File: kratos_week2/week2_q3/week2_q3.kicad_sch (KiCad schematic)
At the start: 17 parts, among them J1 XT60-M, J10 XT60-M, J11 XT60-M, J2 XT60-M, J3 XT60-M, J4 XT60-M, J5 XT60-M, J6 XT60-M, J7 Conn_01x02_Pin, J8 Conn_01x02_Pin, J9 Conn_01x02_Pin

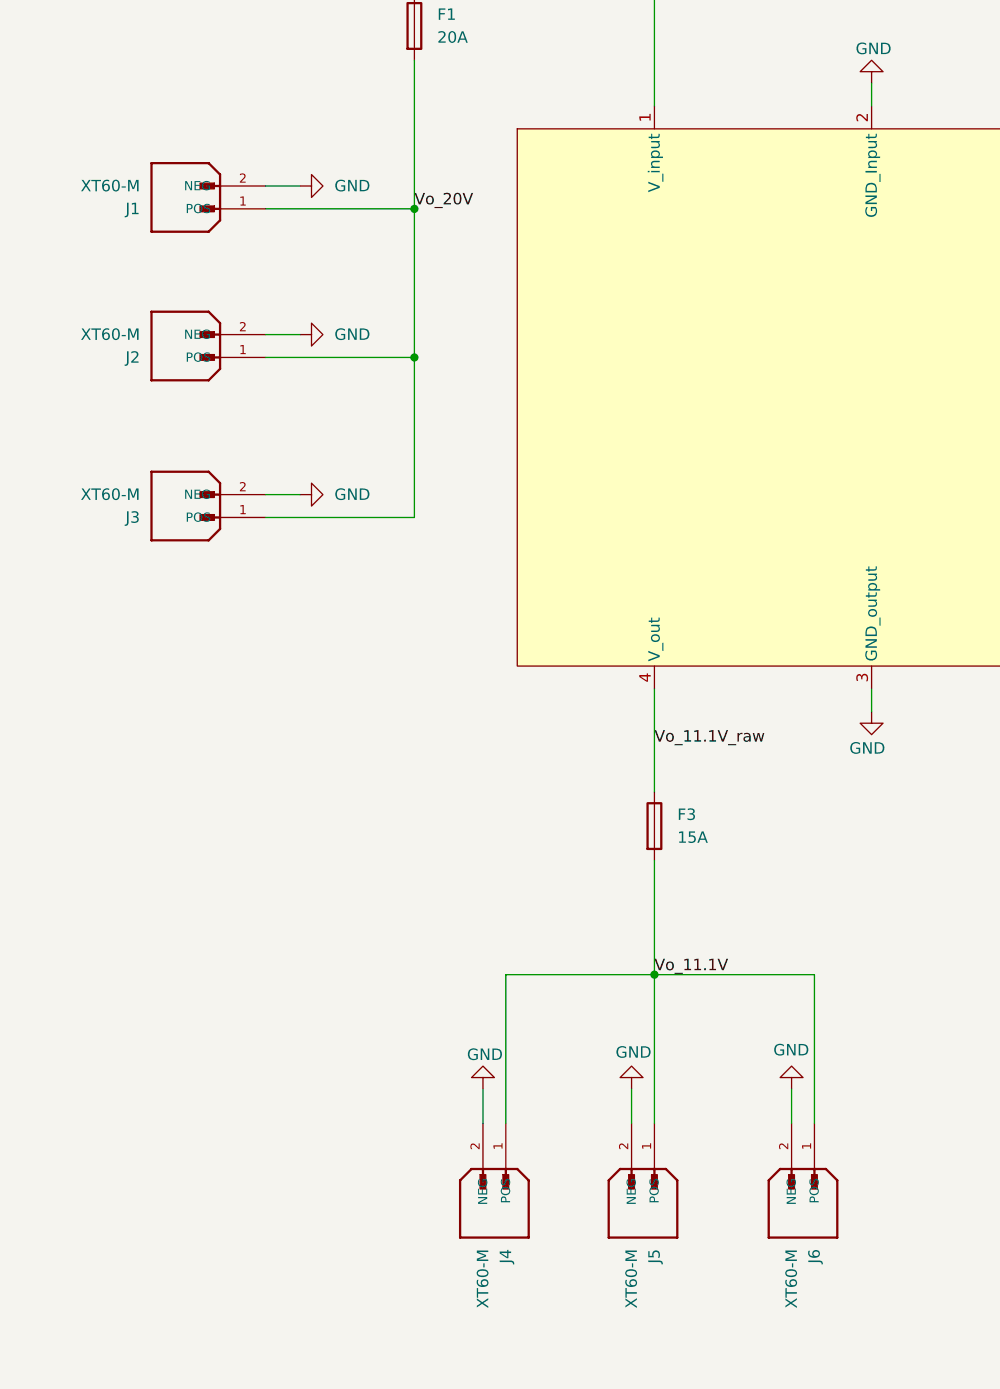
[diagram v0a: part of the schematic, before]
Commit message: Week2_update
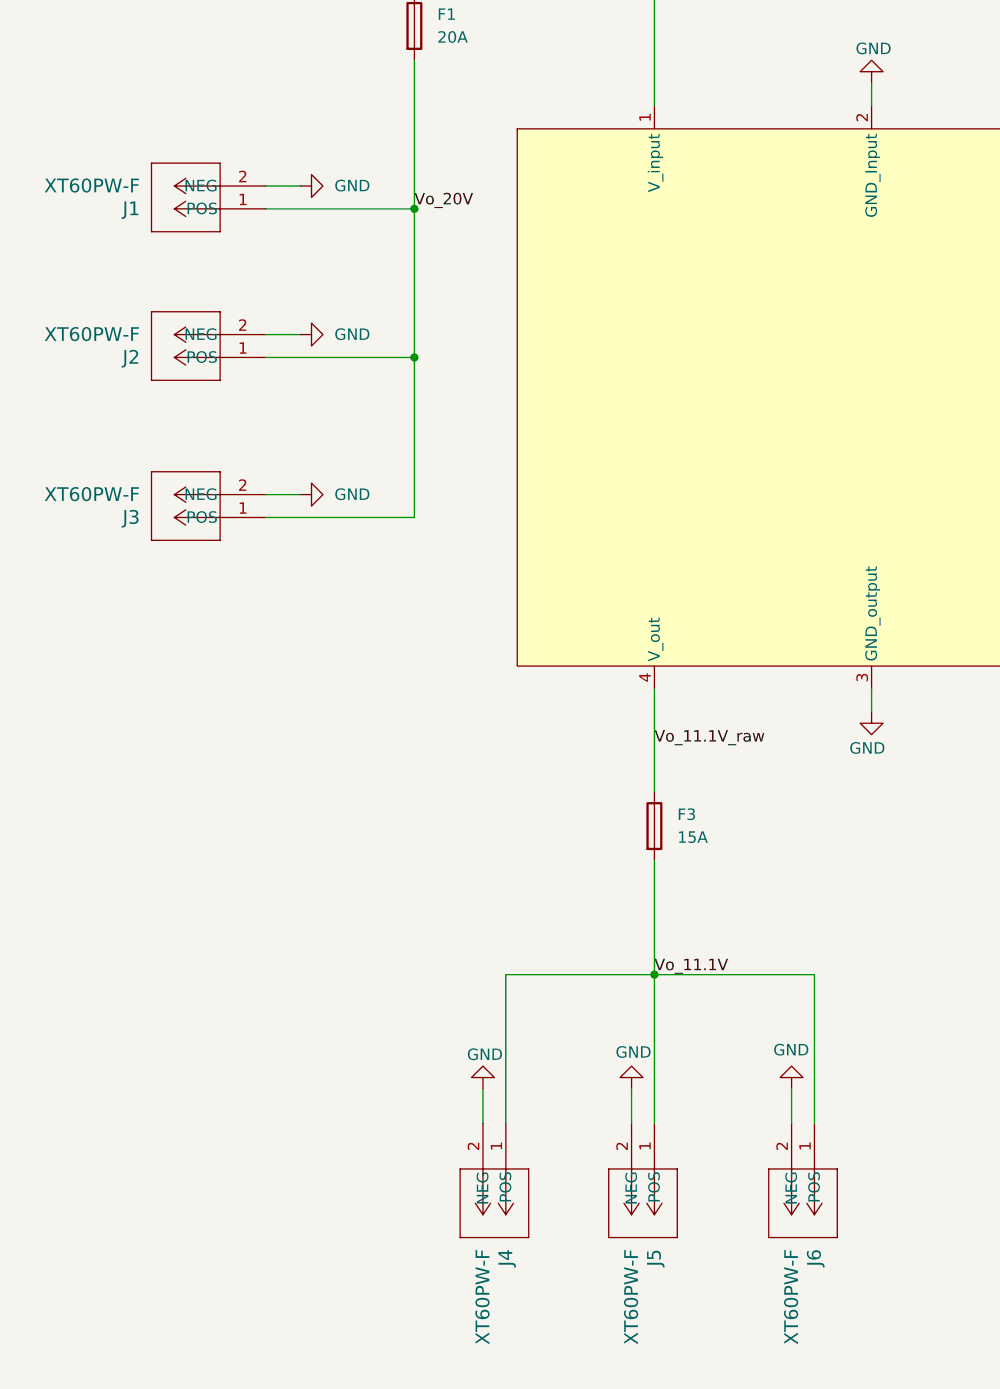
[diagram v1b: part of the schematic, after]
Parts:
- removed J1, J2, J3, J4, J5, J6: XT60-M, Connector_AMASS:AMASS_XT60-M_1x02_P7.20mm_Vertical, symbol XT60-M:XT60-M
- added J1, J2, J3, J4, J5, J6: XT60PW-F, CONN_XT60PW-F_AMA, symbol XT60-M:XT60PW-F
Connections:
- net GND: now also J1.2 (NEG), J2.2 (NEG), J3.2 (NEG), J4.2 (NEG), J5.2 (NEG), J6.2 (NEG)
- net Vo_11.1V: now also J4.1 (POS), J5.1 (POS), J6.1 (POS)
- net Vo_20V: now also J1.1 (POS), J2.1 (POS), J3.1 (POS)
